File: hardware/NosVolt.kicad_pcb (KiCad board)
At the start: 2 copper layers, 100 x 60 mm, 123 parts, among them CN201 100nF, J101 INPUTS, J102 OUTPUTS, J201 BAT_SENSE, J202 BAT_NTC, J801 USB_C_Receptacle_USB2.0_16P, Q501 2N7002, Q502 AO4407A, Q601 2N7002, Q602 AO4407A, Q701 2N7002, Q702 AO4407A, SW101 SW_Reset, SW102 SSSS811101, U101 GMT028-05, U102 ESP32-S3-WROOM-1, U201 ADS1115IDGS, U301 INA226, U401 INA226, U501 INA226, U601 INA226, U701 INA226, U801 AP7361-33ER-13, U802 USBLC6-2SC6, U901 MP2307DN-LF-Z

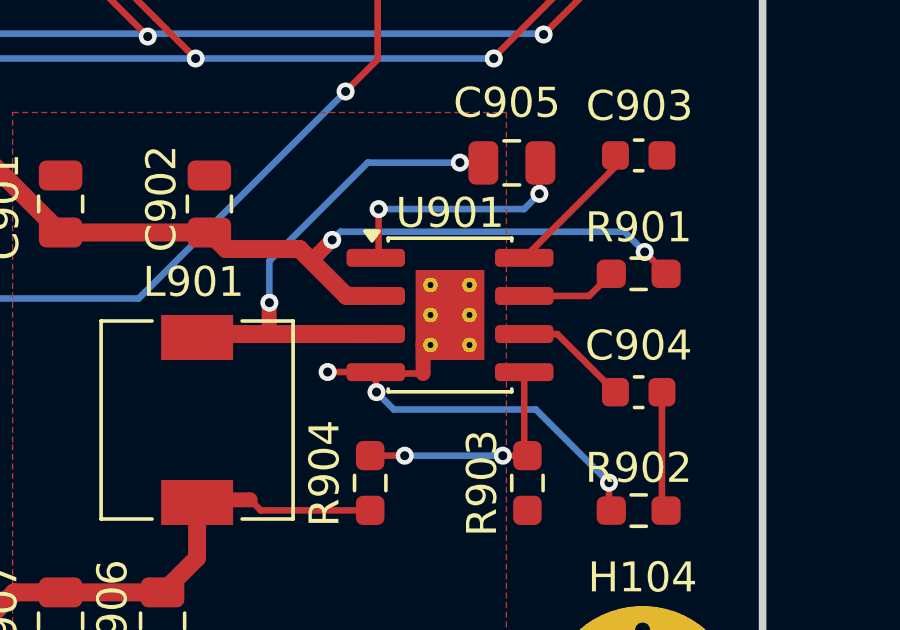
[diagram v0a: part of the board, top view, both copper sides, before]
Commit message: page numbers
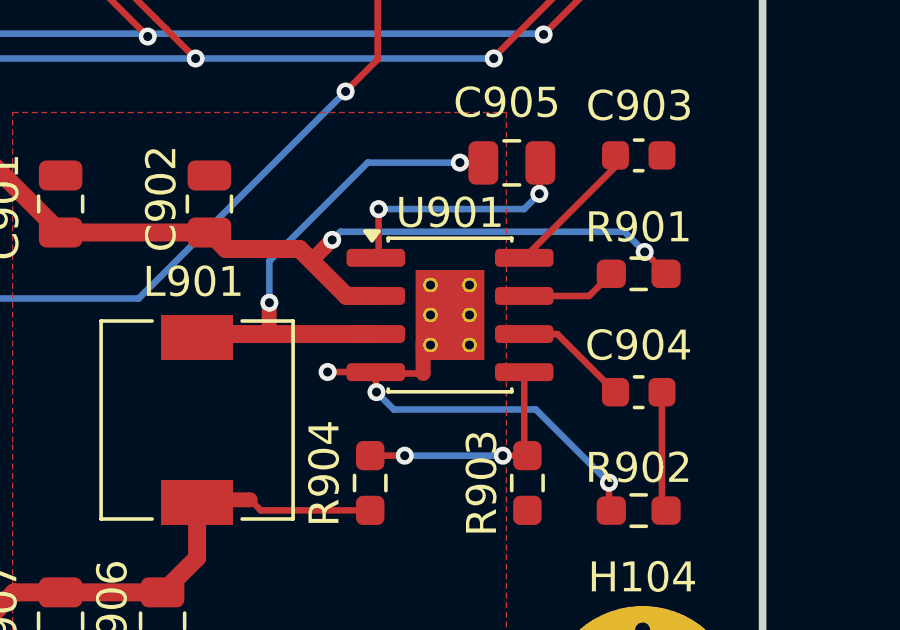
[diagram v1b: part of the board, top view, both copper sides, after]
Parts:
- U901: footprint Package_SO:SOIC-8-1EP_3.9x4.9mm_P1.27mm_EP2.29x3mm_ThermalVias -> NosLib:SOIC-8-1EP_3.9x4.9mm_P1.27mm_EP2.29x3mm_ThermalVias
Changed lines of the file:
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@@
 		(embedded_fonts no)
 	)
-	(footprint "Package_SO:SOIC-8-1EP_3.9x4.9mm_P1.27mm_EP2.29x3mm_ThermalVias"
+	(footprint "NosLib:SOIC-8-1EP_3.9x4.9mm_P1.27mm_EP2.29x3mm_ThermalVias"
 		(layer "F.Cu")
 		(at 192.28 80.55)
@@
 			(pinfunction "GND")
 			(pintype "power_in")
-			(zone_connect 2)
 		)
 		(pad "5" smd roundrect
@@
 			(at -0.65 -1)
 			(size 0.5 0.5)
-			(drill 0.2)
+			(drill 0.3)
+			(property pad_prop_heatsink)
+			(layers "*.Cu" "B.Paste")
+			(remove_unused_layers no)
+			(net 69 "/MP2307/PWR_GND")
+			(pinfunction "EP")
+			(pintype "input")
+		)
+		(pad "9" thru_hole circle
+			(at -0.65 0)
+			(size 0.5 0.5)
+			(drill 0.3)
 			(property pad_prop_heatsink)
 			(layers "*.Cu")
@@
 		)
 		(pad "9" thru_hole circle
-			(at -0.65 0)
-			(size 0.5 0.5)
-			(drill 0.2)
-			(property pad_prop_heatsink)
-			(layers "*.Cu")
-			(remove_unused_layers no)
-			(net 69 "/MP2307/PWR_GND")
-			(pinfunction "EP")
-			(pintype "input")
-		)
-		(pad "9" thru_hole circle
 			(at -0.65 1)
 			(size 0.5 0.5)
-			(drill 0.2)
+			(drill 0.3)
 			(property pad_prop_heatsink)
 			(layers "*.Cu")
@@
 			(at 0.65 -1)
 			(size 0.5 0.5)
-			(drill 0.2)
+			(drill 0.3)
 			(property pad_prop_heatsink)
 			(layers "*.Cu")
@@
 			(at 0.65 0)
 			(size 0.5 0.5)
-			(drill 0.2)
+			(drill 0.3)
 			(property pad_prop_heatsink)
 			(layers "*.Cu")
@@
 			(at 0.65 1)
 			(size 0.5 0.5)
-			(drill 0.2)
+			(drill 0.3)
 			(property pad_prop_heatsink)
 			(layers "*.Cu")
